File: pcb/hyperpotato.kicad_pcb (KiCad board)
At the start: 2 copper layers, 117 x 88.3 mm, 50 parts, among them J1 Conn_01x02_Socket, J2 Conn_01x03_Pin, Q1 AO3401A, SW1 SW_Push_45deg, SW10 SW_Push_45deg, SW11 SW_Push_45deg, SW12 SW_Push_45deg, SW13 SW_Push_45deg, SW14 SW_SPDT, SW15 SW_Push, SW2 SW_Push_45deg, SW3 SW_Push_45deg, SW4 SW_Push_45deg, SW5 SW_Push_45deg, SW6 SW_Push_45deg, SW7 SW_Push_45deg, SW8 SW_Push_45deg, SW9 SW_Push_45deg, U1 Seeeduino Xiao nRF52840, U2 SK8707-01-SENSOR, U3 SK8707-01, U4 DRV2605LDGS, U5 74HC595

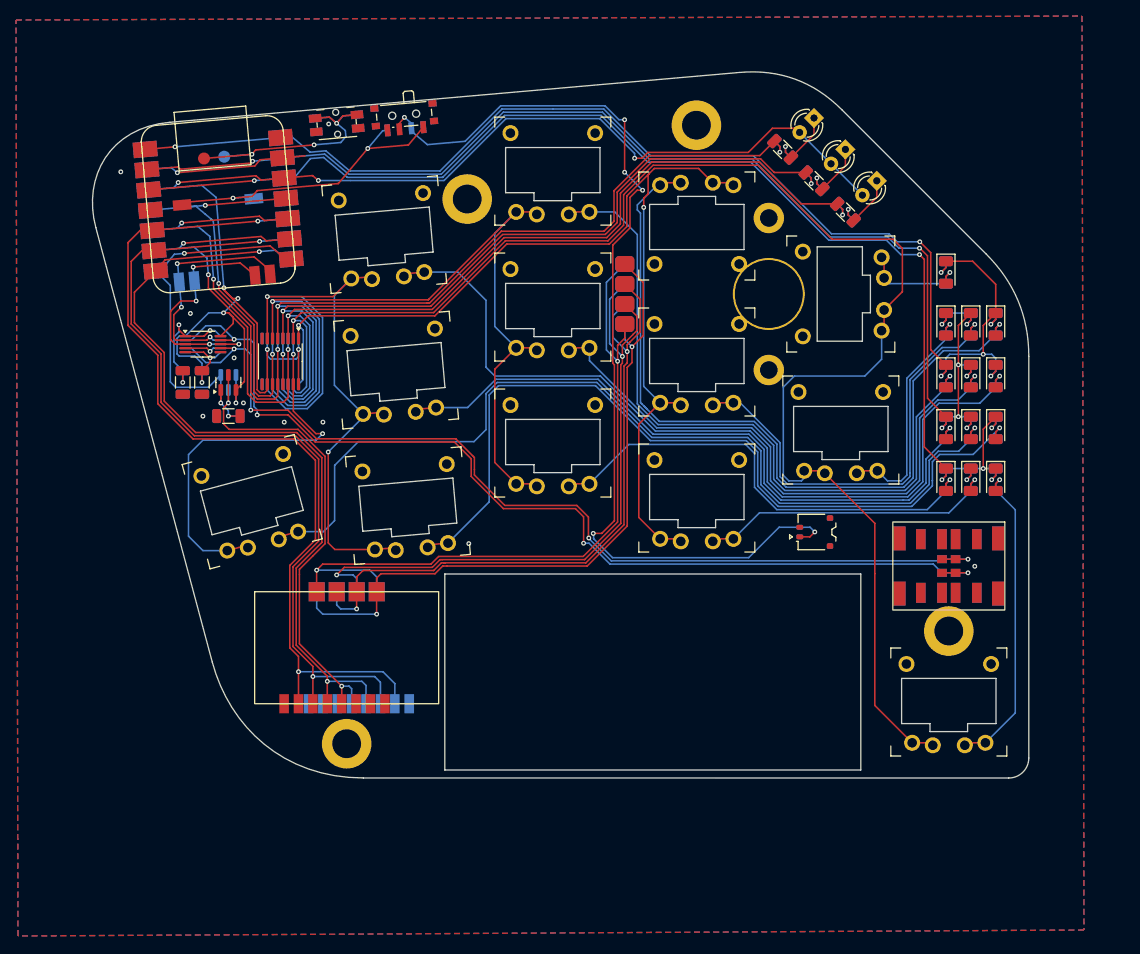
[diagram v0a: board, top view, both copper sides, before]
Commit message: Ready to go!
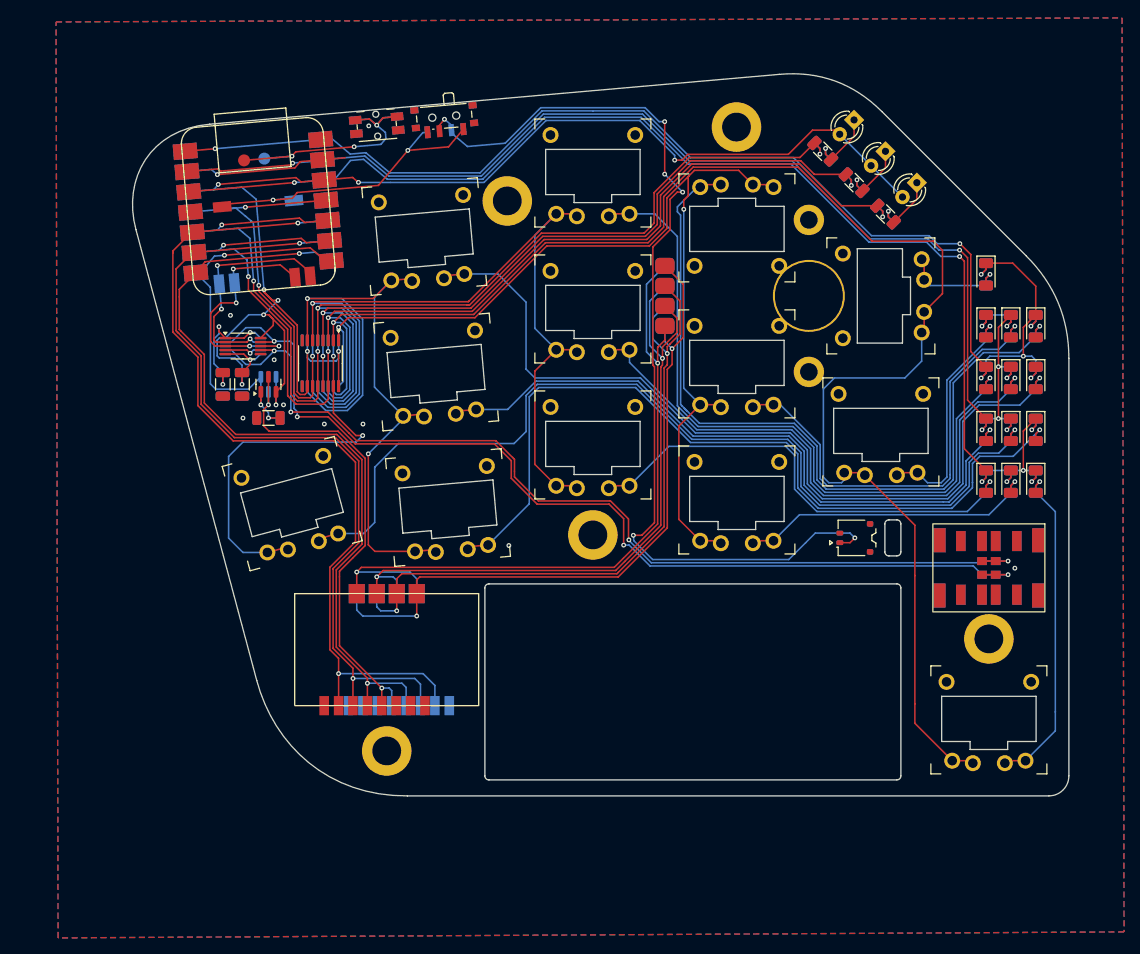
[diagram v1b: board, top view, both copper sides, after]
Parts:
- added H2: MountingHole, hyperpotato:MountingHole, F.Cu at (203.3, 129.4)
- moved SW13 5.49 mm to (252.8, 152.5)
- moved H5 5.10 mm to (252.8, 142.4)
- moved H3 5.09 mm to (177.5, 156.4)
- moved J1 5.06 mm to (236.0, 129.8)
- moved C2 5.01 mm to (157.0, 110.6)
- moved D1 5.01 mm to (258.6, 109.8)
- moved D16 5.01 mm to (243.8, 85.4)
- moved H1 5.01 mm to (230.3, 99.5)
- moved R3 5.01 mm to (235.9, 85.4)
- moved SW5 5.01 mm to (165.7, 125.5)
- moved SW9 5.01 mm to (239.3, 116.5)
- moved D3 5.01 mm to (258.6, 103.3)
- moved D6 5.01 mm to (252.4, 116.3)
- moved D7 5.01 mm to (255.5, 109.8)
- moved H6 5.01 mm to (221.2, 78.4)
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- renumbered H7 to H5
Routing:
- net Net-(D13-A): track 39.5 -> 41.9 mm
- net COL4: track 191.2 -> 193.6 mm
- net TP_GND: track 81.9 -> 84.0 mm
- net TP_DATA: track 113.2 -> 111.9 mm
- net TP_CLK: track 107.4 -> 106.5 mm
- net GND: vias 14 -> 13
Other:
- board size 117 x 88.3 mm -> 117 x 90.3 mm
